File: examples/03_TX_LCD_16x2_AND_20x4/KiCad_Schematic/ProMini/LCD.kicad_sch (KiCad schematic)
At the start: 9 parts, among them J1 KIT DIY 5~7W QN8066, U1 LCD 16x02 or 20x04

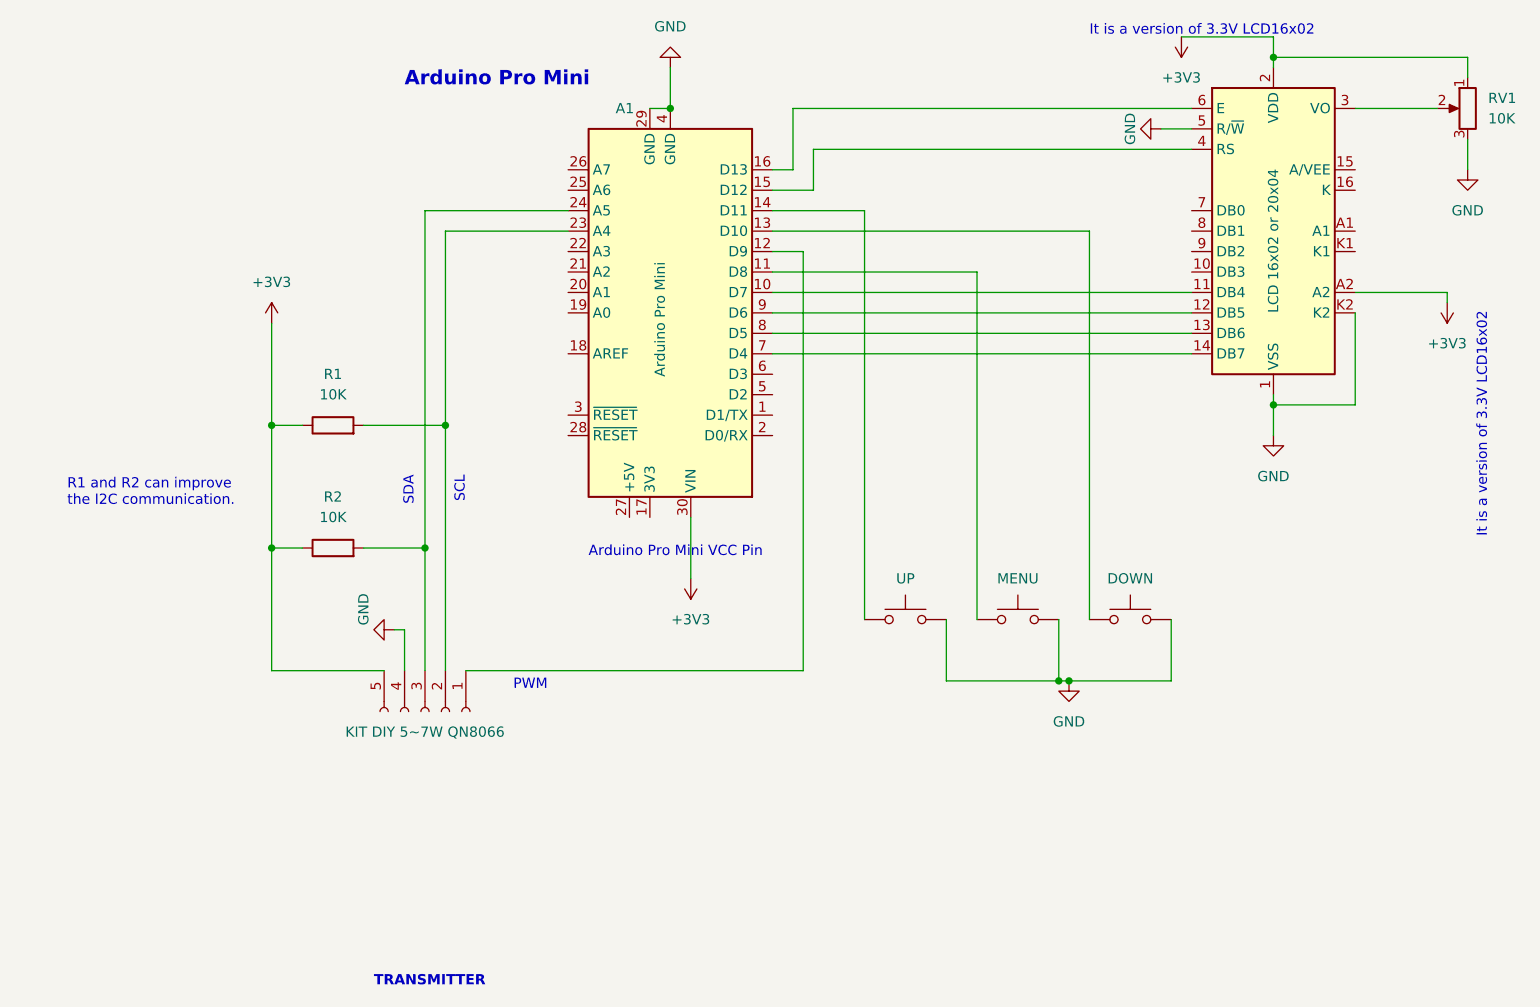
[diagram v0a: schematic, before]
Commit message: Doc
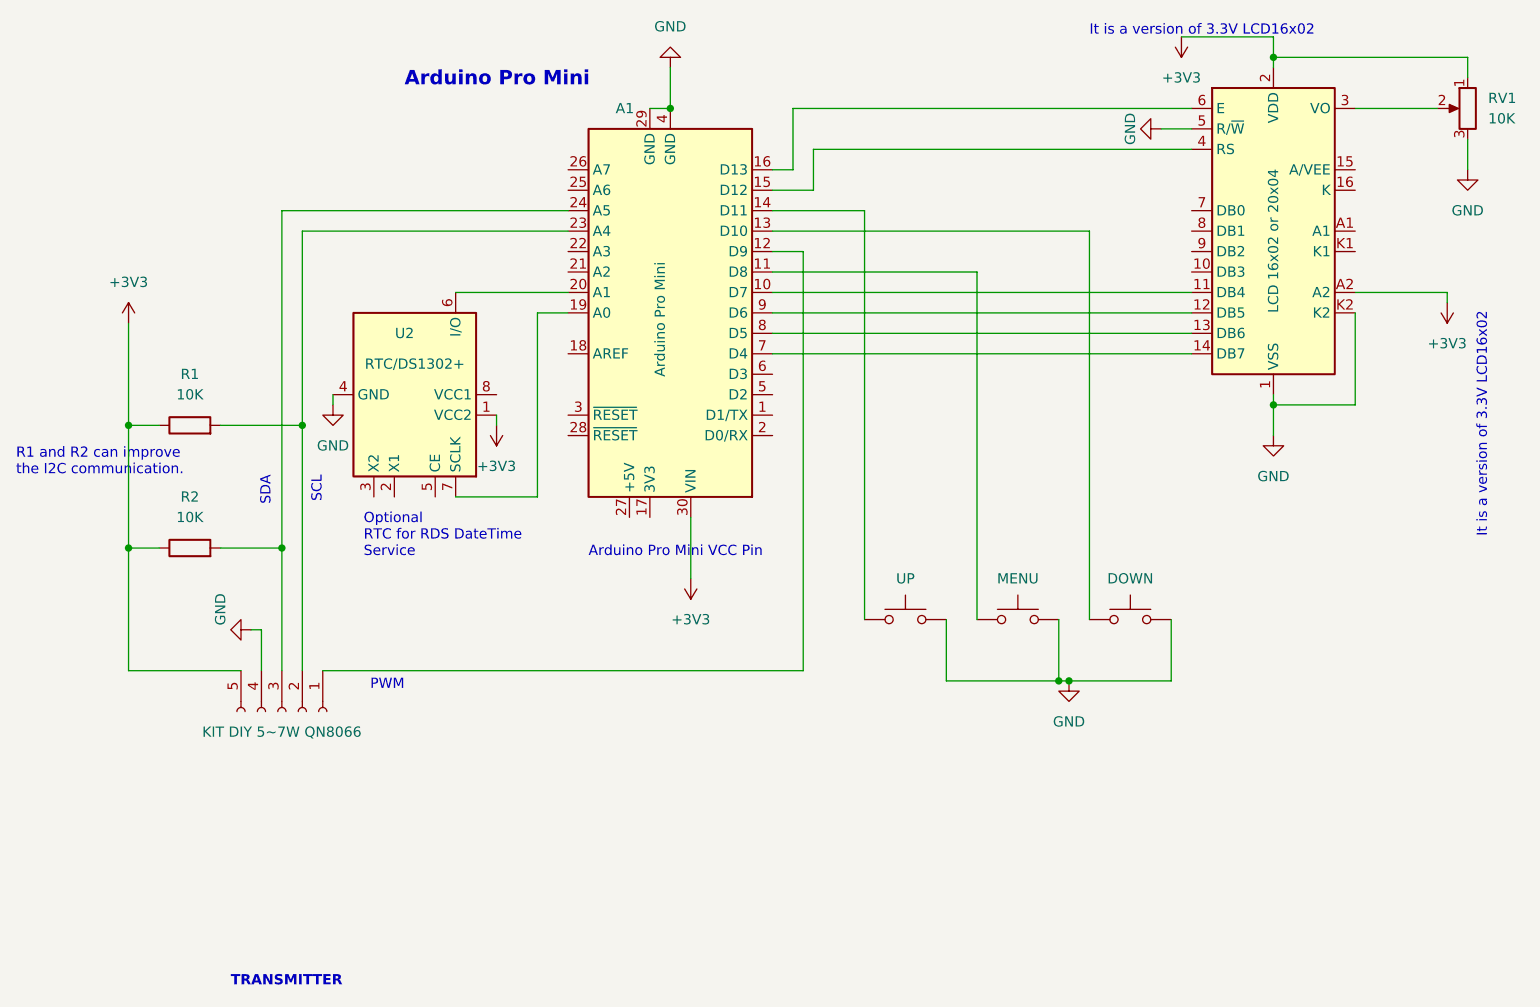
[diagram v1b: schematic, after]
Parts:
- added U2: RTC/DS1302+, Package_DIP:DIP-8_W7.62mm, symbol Timer_RTC:DS1302+
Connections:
- net +3V3: now also U2.1 (VCC2)
- net GND: now also U2.4 (GND)
- net at A1.19 (A0): now also U2.7 (SCLK)
- net at A1.20 (A1): now also U2.6 (I/O)
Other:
- note added: "Optional RTC for RDS DateTime Service"
- moved on the sheet: R1, R2
